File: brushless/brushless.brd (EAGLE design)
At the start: 30 x 48 mm, 71 parts, among them Q1 BUK7Y12-40E, Q2 BUK7Y12-40E, Q3 BUK7Y12-40E, Q4 BUK7Y12-40E, Q5 BUK7Y12-40E, Q6 BUK7Y12-40E, X2 MOTOR

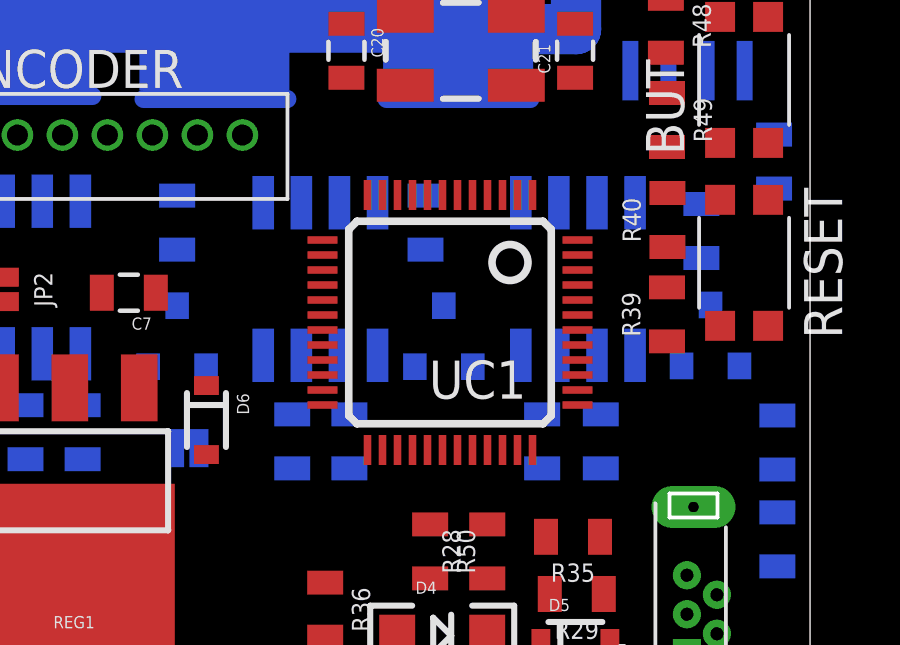
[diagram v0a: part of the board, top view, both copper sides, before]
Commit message: 0.25
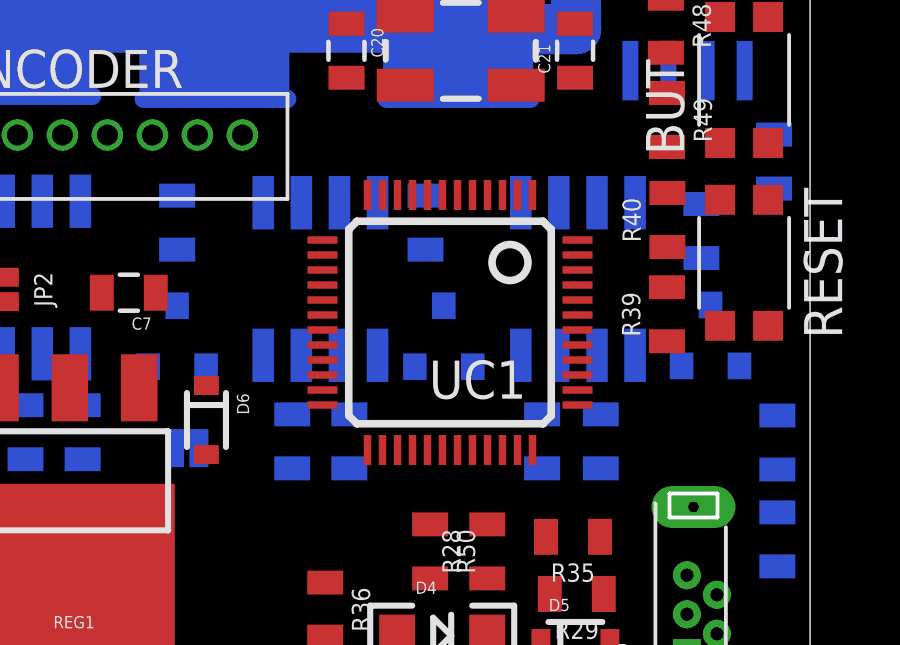
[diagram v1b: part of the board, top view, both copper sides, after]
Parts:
- UC1: device stm32:LQFP48 -> rhoban:STM32_LQFP48
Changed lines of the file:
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@@
 <attribute name="FARNELL" value="1581233" x="17.6578" y="2.5118" size="1.778" layer="27" display="off"/>
 </element>
-<element name="UC1" library="stm32" package="LQFP48" value="STM32F103CBT6" x="17.9182" y="12.951" rot="R180">
+<element name="UC1" library="rhoban" package="STM32_LQFP48" value="STM32F103CBT6" x="17.9182" y="12.951" rot="R180">
 <attribute name="FARNELL" value="1606327" x="17.9182" y="12.951" size="1.778" layer="27" rot="R180" display="off"/>
 </element>
